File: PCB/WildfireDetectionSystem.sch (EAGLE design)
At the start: 101 parts, among them IC1 STM32L476RGT6, J1 10118192-0001LF, J3 B4B-XH-A, J4 B5B-XH-A, J7 B4B-PH-K-S, J8 U.FL-R-SMT-1(10), J9 B2B-PH-K-S, SW1 434133025816, U1 BME280, U3 NEO-6M-GPS, U4 TPS62142RGTT, U5 TPS61022RWUR, U6 LMR33630ADDA, U7 BQ24074RGTR, Y1 ABLS-8.000MHZ-B2-T, Y2 ECS-.327-12.5-12QS-TR

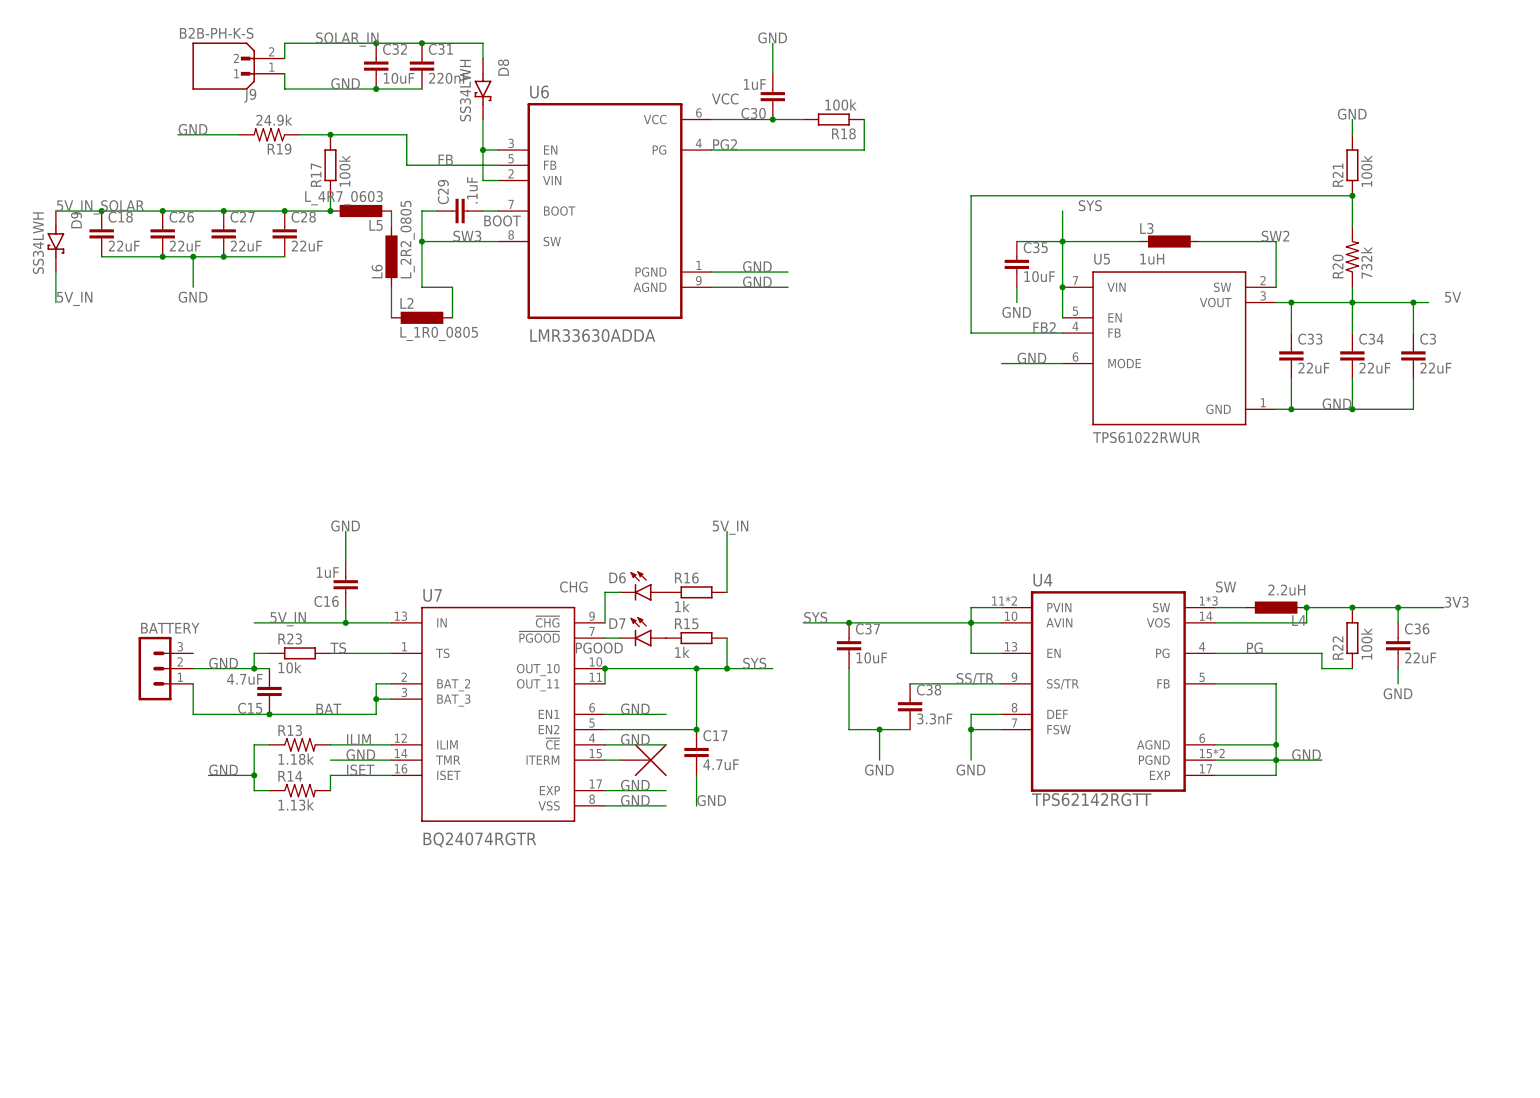
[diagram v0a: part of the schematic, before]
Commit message: pcbv2
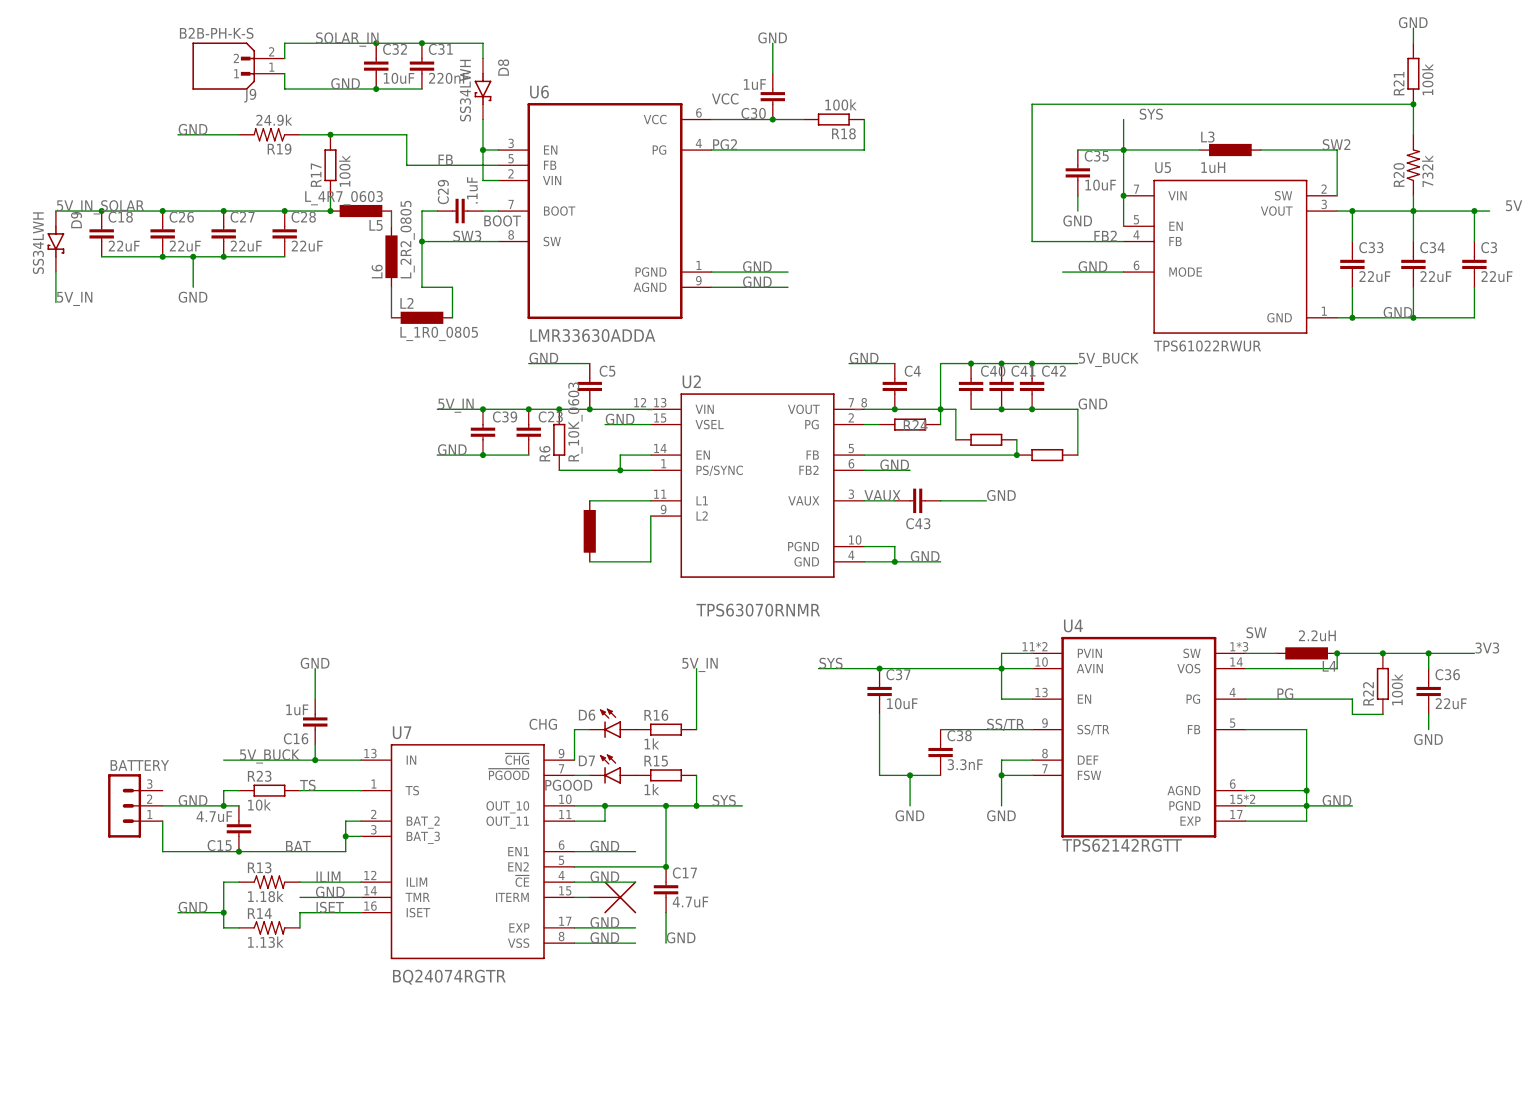
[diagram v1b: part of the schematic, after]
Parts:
- added C23, C39: C_10UF/25V_0805, JLC PCB Basic Parts_loc:C_10UF/25V_0805
- added C4, C5: C_10UF/10V_0603, JLC PCB Basic Parts_loc:C_10UF/10V_0603
- added C40, C41, C42: C_22UF/25V_0805, JLC PCB Basic Parts_loc:C_22UF/25V_0805
- added C43: C_100NF/50V_0603, JLC PCB Basic Parts_loc:C_100NF/50V_0603
- added L8: L_1R0_0805, JLC PCB Basic Parts_loc:L_1R0_0805
- added R24: R_100K_0603, JLC PCB Basic Parts_loc:R_100K_0603
- added R25: R_680K_0603, JLC PCB Basic Parts_loc:R_680K_0603
- added R26: R_130K_0603, JLC PCB Basic Parts_loc:R_130K_0603
- added R6: R_10K_0603, JLC PCB Basic Parts_loc:R_10K_0603
- added U2: TPS63070RNMR, TPS63070RNMR:TPS63070RNMR
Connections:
- new net 5V_BUCK: C16.1, C4.2, C40.1, C41.1, C42.1, R24.2, R25.1, U2.VOUT, U7.IN
- new net N$19: L8.1, U2.L1
- new net N$20: L8.2, U2.L2
- new net N$21: R6.1, U2.EN, U2.PS/SYNC
- new net N$22: R24.1, U2.PG
- new net N$23: R25.2, R26.2, U2.FB
- new net VAUX: C43.1, U2.VAUX
- net 5V_IN: now also C23.1, C39.1, C5.2, R6.2, U2.VIN; no longer C16.1, U7.IN
- net GND: now also C23.2, C39.2, C4.1, C40.2, C41.2, C42.2, C43.2, C5.1, R26.1, U2.FB2, U2.GND, U2.PGND, U2.VSEL
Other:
- moved on the sheet: BATTERY, C15, C16, C17, C3, C33, C34, C35, C36, C37, C38, D6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
